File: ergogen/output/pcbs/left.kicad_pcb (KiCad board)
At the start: 2 copper layers, 129.3 x 92.4 mm, 59 parts

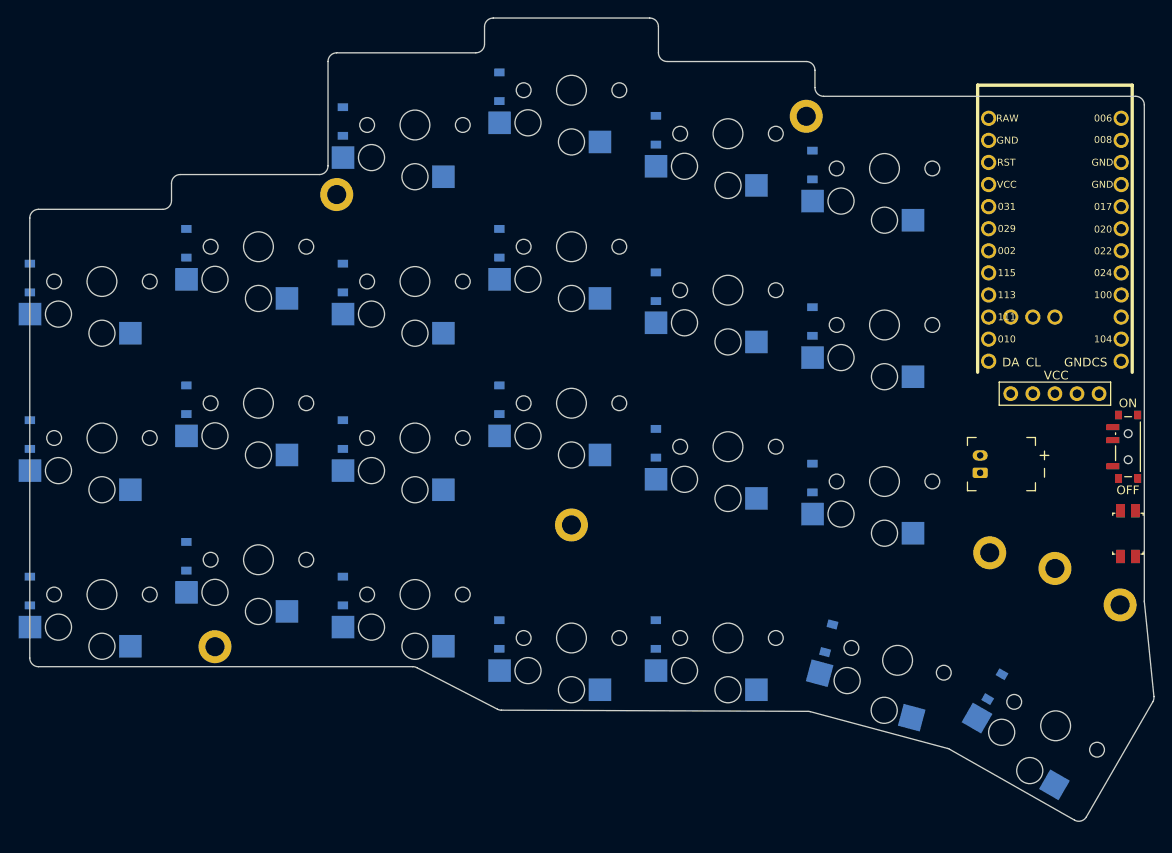
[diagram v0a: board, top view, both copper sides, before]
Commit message: wip: unrouted v2
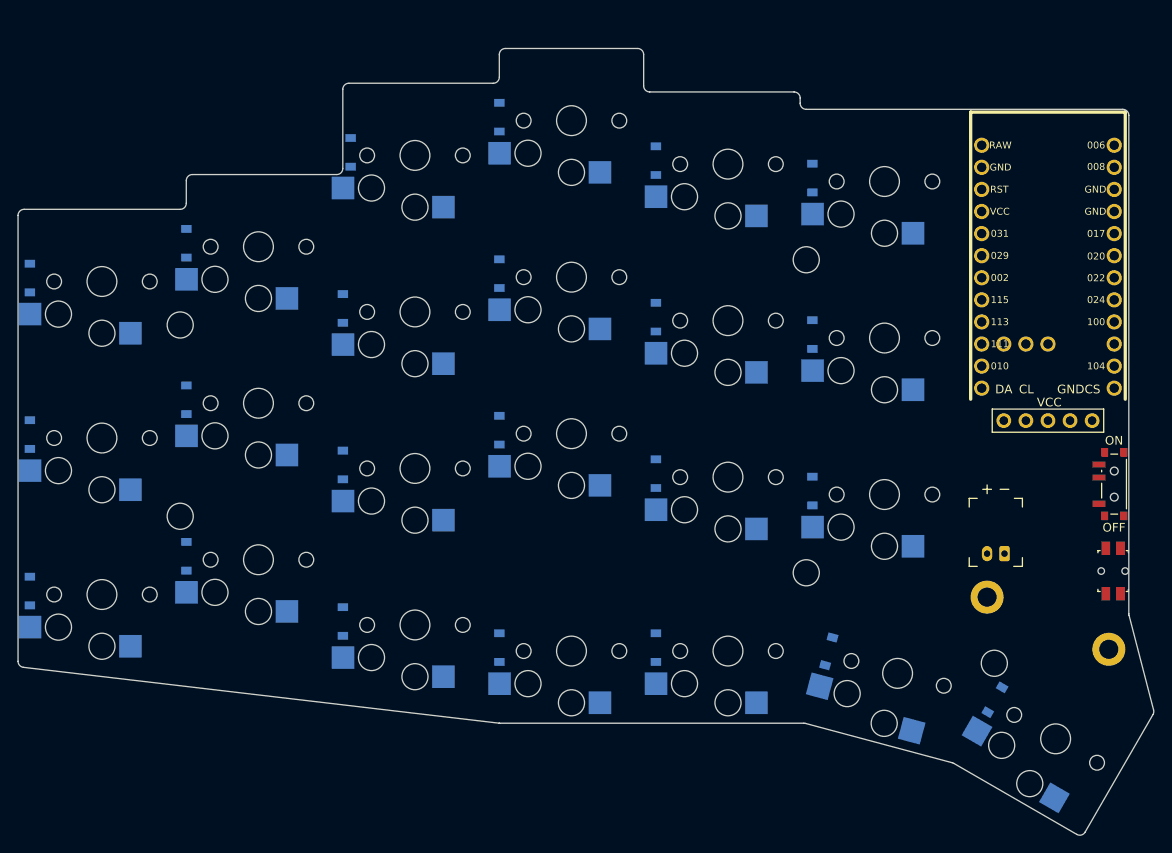
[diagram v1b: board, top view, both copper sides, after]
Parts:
- removed H3, H4, H5, H6, H7: , ceoloide:mounting_hole_plated
- added MH1: , ceoloide:mounting_hole_npth, F.Cu at (251.0, 133.5)
- added MH2: , ceoloide:mounting_hole_npth, F.Cu at (179.0, 141.0)
- added MH3: , ceoloide:mounting_hole_npth, F.Cu at (179.0, 163.0)
- added MH4: , ceoloide:mounting_hole_npth, F.Cu at (251.0, 169.5)
- added MH5: , ceoloide:mounting_hole_npth, F.Cu at (272.6, 179.9)
- moved G 123.3 mm to (278.8, 160.3)
- moved H2 103.1 mm to (285.8, 178.3)
- moved D23 96.3 mm to (198.6, 121.2), turned to -90 degrees
- moved D19 66.2 mm to (215.7, 178.1)
- moved H1 59.1 mm to (271.8, 172.3)
- moved D13 48.0 mm to (233.7, 158.1)
- moved D16 45.2 mm to (251.7, 160.1)
- moved D10 39.8 mm to (215.7, 153.1)
- moved D22 20.4 mm to (272.7, 184.1), turned to -120 degrees
- moved D21 20.0 mm to (253.6, 178.5), turned to -105 degrees
- moved D20 18.1 mm to (233.7, 178.1)
- moved D17 16.5 mm to (251.7, 142.1)
- moved D18 16.5 mm to (251.7, 124.1)
- moved D11 14.5 mm to (215.7, 135.1)
- moved D12 14.5 mm to (215.7, 117.1)
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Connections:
- D10 pad 1: P017 -> P022
- D10 pad 2: ring_top -> middle_bottom
- D11 pad 1: P022 -> P020
- D11 pad 2: middle_bottom -> middle_home
- D12 pad 1: P020 -> P017
- D12 pad 2: middle_home -> middle_top
- D13 pad 1: P017 -> P022
- D13 pad 2: middle_top -> index_bottom
- D14 pad 1: P022 -> P020
- D14 pad 2: index_bottom -> index_home
- D15 pad 1: P020 -> P017
- D15 pad 2: index_home -> index_top
- D16 pad 1: P017 -> P022
- D16 pad 2: index_top -> inner_bottom
- D17 pad 1: P022 -> P020
- D17 pad 2: inner_bottom -> inner_home
- D18 pad 1: P020 -> P017
- D18 pad 2: inner_home -> inner_top
- D19 pad 1: P017 -> P024
- D19 pad 2: inner_top -> inner_thumb
- D20 pad 2: inner_thumb -> close_thumb
- D21 pad 2: close_thumb -> home_thumb
- D22 pad 2: home_thumb -> outer_thumb
- D23 pad 1: P024 -> P017
- D23 pad 2: outer_thumb -> ring_top
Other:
- board size 129.3 x 92.4 mm -> 130.6 x 90.5 mm
